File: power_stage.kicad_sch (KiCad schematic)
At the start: 32 parts, among them J1 Input, J1 Output, Q1 IMW120R014M1H, Q2 IMW120R014M1H, Q6 2N7002BK,215, U4 TC4432VOA

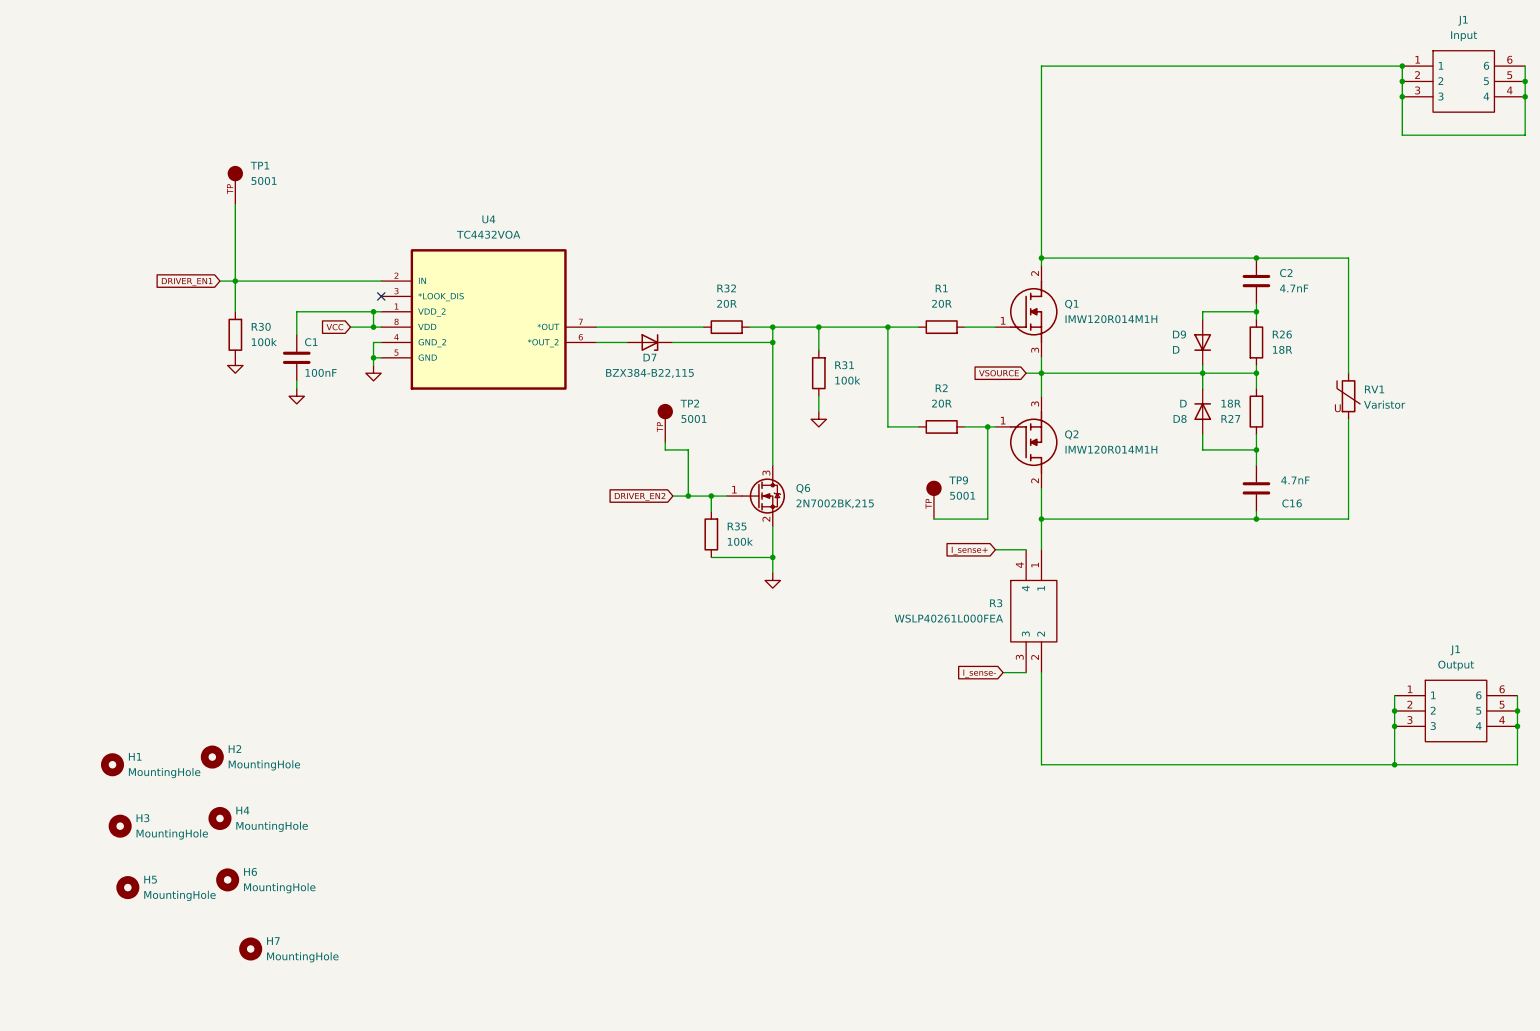
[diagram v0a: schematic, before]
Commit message: Final Design
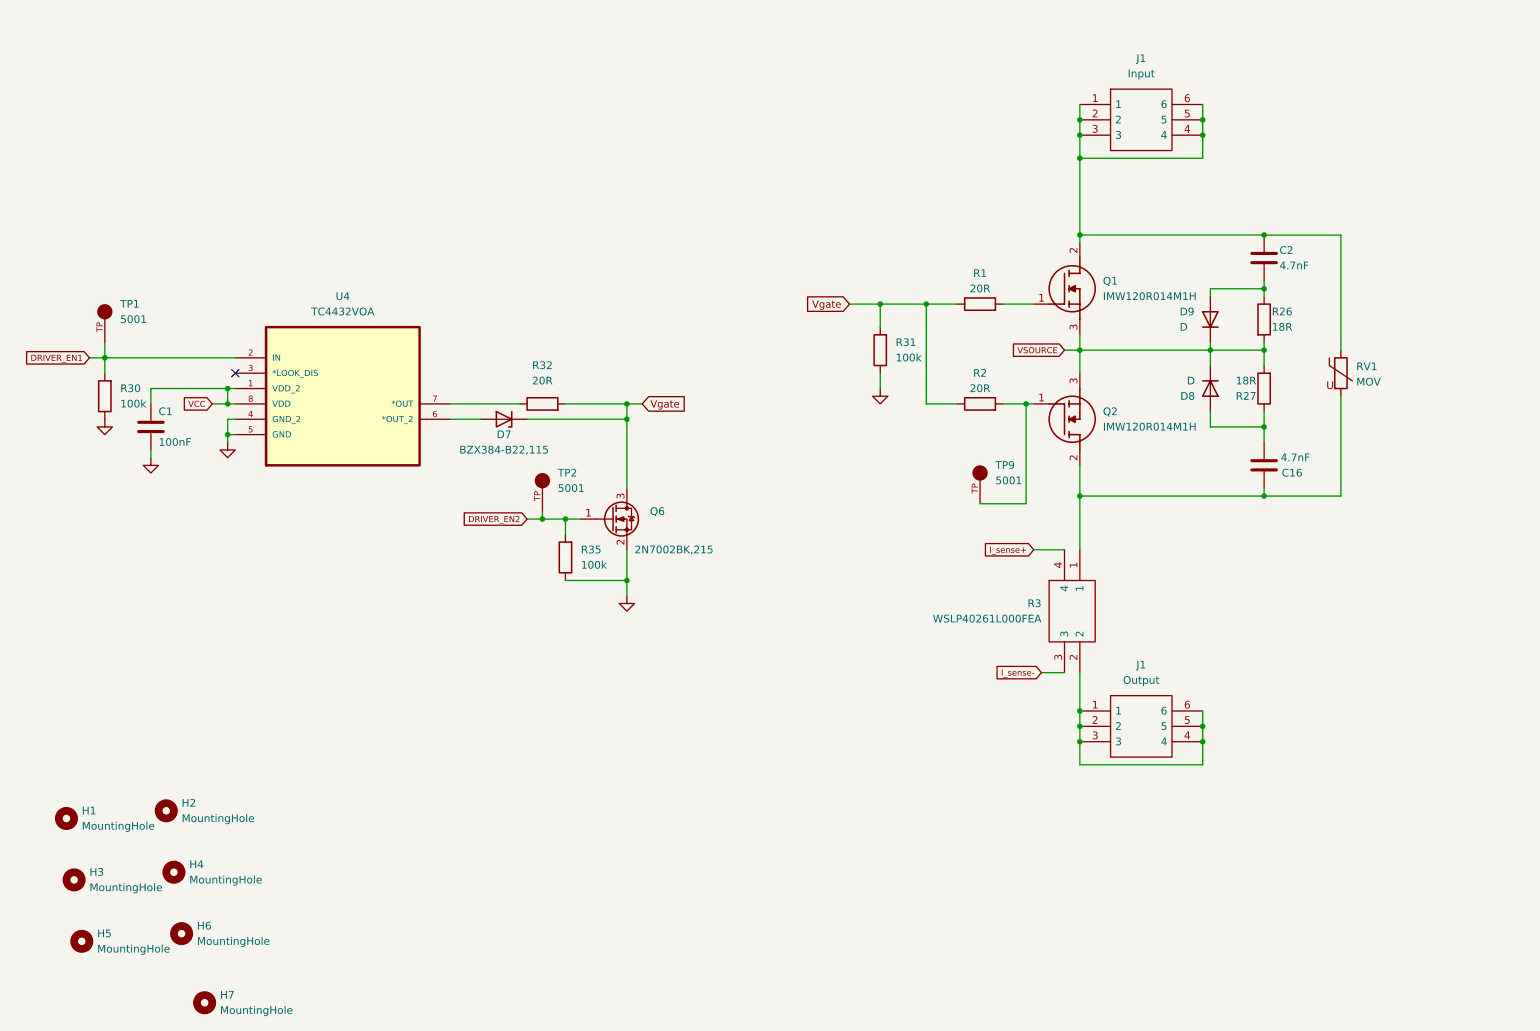
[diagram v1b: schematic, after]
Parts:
- RV1: value Varistor -> MOV
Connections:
- net Vgate: now reaches D7.1 (K), Q6.3 (D), R1.1, R2.1, R31.2, R32.2
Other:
- moved on the sheet: C1, C16, C2, D7, D8, D9, H1, H2, H3, H4, H5, H6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
